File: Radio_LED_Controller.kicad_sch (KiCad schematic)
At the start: 15 parts, among them J1 Conn_01x04_Pin, J2 Conn_01x03_Pin, J3 Conn_01x05, J4 UPDI, J5 Conn_01x02_Pin, J6 Conn_01x02_Pin, J7 Conn_01x05, J8 Conn_01x03_Pin, J9 Conn_01x03_Pin, Q2 SS8050, Q3 SS8050, U1 ATtiny816-M

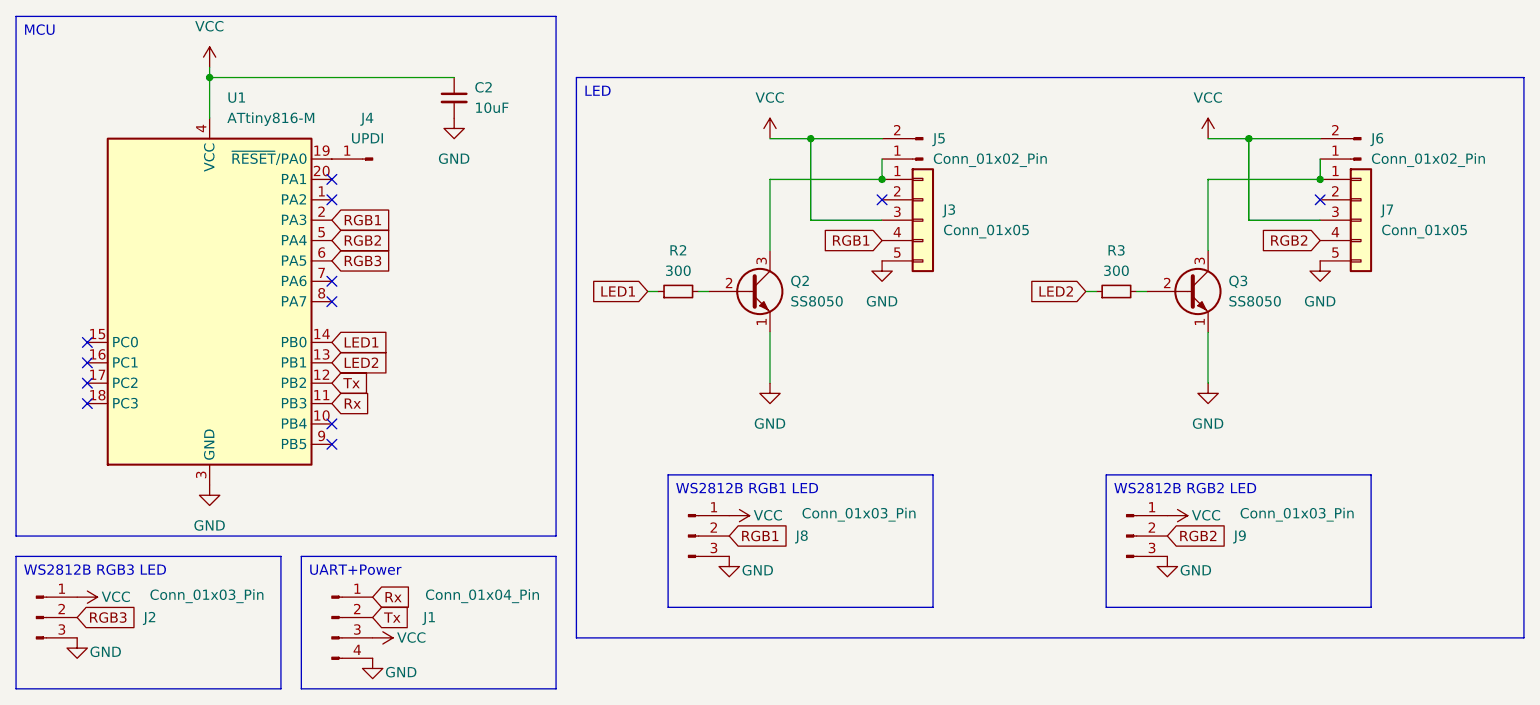
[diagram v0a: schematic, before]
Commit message: v0.2
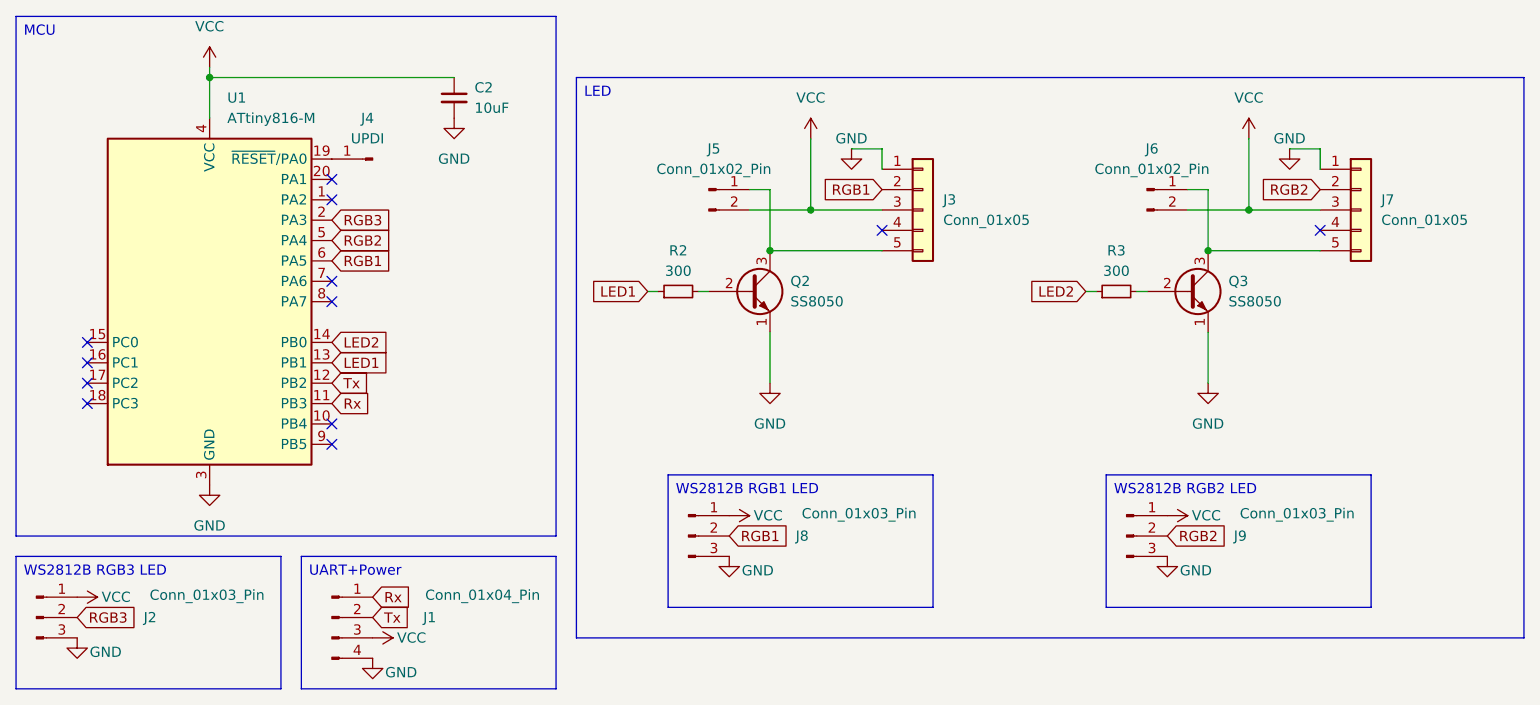
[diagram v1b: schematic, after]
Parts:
- J3, J7: footprint Connector_JST:JST_GH_SM05B-GHS-TB_1x05-1MP_P1.25mm_Horizontal -> Connector_Molex:Molex_PicoBlade_53261-0571_1x05-1MP_P1.25mm_Horizontal
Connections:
- net GND: now also J3.1 (Pin_1), J7.1 (Pin_1); no longer J3.5 (Pin_5), J7.5 (Pin_5)
- net LED1: now also U1.13 (PB1); no longer U1.14 (PB0)
- net LED2: now also U1.14 (PB0); no longer U1.13 (PB1)
- net RGB1: now also J3.2 (Pin_2), U1.6 (PA5); no longer J3.4 (Pin_4), U1.2 (PA3)
- net RGB2: now also J7.2 (Pin_2); no longer J7.4 (Pin_4)
- net RGB3: now also U1.2 (PA3); no longer U1.6 (PA5)
- net at J6.1 (Pin_1), Q3.3 (C): now also J7.5 (Pin_5); no longer J7.1 (Pin_1)
- net at J5.1 (Pin_1), Q2.3 (C): now also J3.5 (Pin_5); no longer J3.1 (Pin_1)
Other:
- moved on the sheet: J3, J5, J6, J7
